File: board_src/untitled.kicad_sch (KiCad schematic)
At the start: 3 parts, among them J3 Conn_01x03, U5 DS18B20

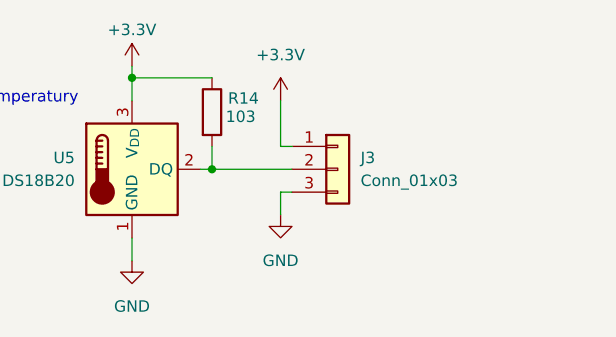
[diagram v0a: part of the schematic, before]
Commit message: Wersja początkowa 9.0
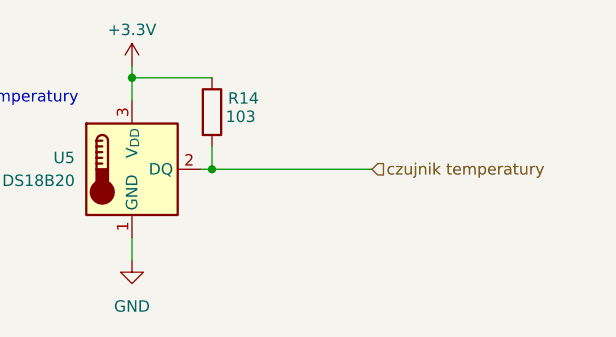
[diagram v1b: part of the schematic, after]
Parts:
- removed J3: Conn_01x03, symbol Connector_Generic:Conn_01x03
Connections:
- net czujnik temperatury: now reaches R14.2, U5.2 (DQ)
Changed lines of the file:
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@@
 	(wire
 		(pts
-			(xy 119.38 93.98) (xy 119.38 88.9)
-		)
-		(stroke
-			(width 0)
-			(type default)
-		)
-	)
-	(wire
-		(pts
-			(xy 120.65 99.06) (xy 119.38 99.06)
-		)
-		(stroke
-			(width 0)
-			(type default)
-		)
-	)
-	(wire
-		(pts
-			(xy 111.76 96.52) (xy 120.65 96.52)
+			(xy 111.76 96.52) (xy 129.54 96.52)
 		)
 		(stroke
@@
 	(wire
 		(pts
-			(xy 119.38 99.06) (xy 119.38 101.6)
-		)
-		(stroke
-			(width 0)
-			(type default)
-		)
-	)
-	(wire
-		(pts
-			(xy 120.65 93.98) (xy 119.38 93.98)
-		)
-		(stroke
-			(width 0)
-			(type default)
-		)
-	)
-	(wire
-		(pts
 			(xy 111.76 93.98) (xy 111.76 96.52)
 		)
@@
 			(width 0)
 			(type default)
+		)
+	)
+	(hierarchical_label "czujnik temperatury"
+		(shape input)
+		(at 129.54 96.52 0)
+		(effects
+			(font
+				(size 1.27 1.27)
+			)
+			(justify left)
 		)
 	)
@@
 	)
 	(symbol
-		(lib_id "Connector_Generic:Conn_01x03")
-		(at 125.73 96.52 0)
-		(unit 1)
-		(exclude_from_sim no)
-		(in_bom yes)
-		(on_board yes)
-		(dnp no)
-		(fields_autoplaced yes)
-		(property "Reference" "J3"
-			(at 128.27 95.2499 0)
-			(effects
-				(font
-					(size 1.27 1.27)
-				)
-				(justify left)
-			)
-		)
-		(property "Value" "Conn_01x03"
-			(at 128.27 97.7899 0)
-			(effects
-				(font
-					(size 1.27 1.27)
-				)
-				(justify left)
-			)
-		)
-		(property "Footprint" ""
-			(at 125.73 96.52 0)
-			(effects
-				(font
-					(size 1.27 1.27)
-				)
-				(hide yes)
-			)
-		)
-		(property "Datasheet" "~"
-			(at 125.73 96.52 0)
-			(effects
-				(font
-					(size 1.27 1.27)
-				)
-				(hide yes)
-			)
-		)
-		(property "Description" "Generic connector, single row, 01x03, script generated (kicad-library-utils/schlib/autogen/connector/)"
-			(at 125.73 96.52 0)
-			(effects
-				(font
-					(size 1.27 1.27)
-				)
-				(hide yes)
-			)
-		)
-		(pin "3"
-		)
-		(pin "2"
-		)
-		(pin "1"
-		)
-		(instances
-			(project "board"
-				(path "/772e9f49-cfcf-4cf6-843d-0684684f2d4b/4ce4dd53-34e3-426c-821d-561d412e5bd5"
-					(reference "J3")
-					(unit 1)
-				)
-			)
-		)
-	)
-	(symbol
 		(lib_id "power:GND")
 		(at 102.87 106.68 0)
@@
 					(unit 1)
 				)
-			)
-		)
-	)
-	(symbol
-		(lib_id "power:GND")
-		(at 119.38 101.6 0)
-		(unit 1)
-		(exclude_from_sim no)
-		(in_bom yes)
-		(on_board yes)
-		(dnp no)
-		(fields_autoplaced yes)
-		(property "Reference" "#PWR019"
-			(at 119.38 107.95 0)
-			(effects
-				(font
-					(size 1.27 1.27)
-				)
-				(hide yes)
-			)
-		)
-		(property "Value" "GND"
-			(at 119.38 106.68 0)
-			(effects
-				(font
-					(size 1.27 1.27)
-				)
-			)
-		)
-		(property "Footprint" ""
-			(at 119.38 101.6 0)
-			(effects
-				(font
-					(size 1.27 1.27)
-				)
-				(hide yes)
-			)
-		)
-		(property "Datasheet" ""
-			(at 119.38 101.6 0)
-			(effects
-				(font
-					(size 1.27 1.27)
-				)
-				(hide yes)
-			)
-		)
-		(property "Description" "Power symbol creates a global label with name \"GND\" , ground"
-			(at 119.38 101.6 0)
-			(effects
-				(font
-					(size 1.27 1.27)
-				)
-				(hide yes)
-			)
-		)
-		(pin "1"
-		)
-		(instances
-			(project "board"
-				(path "/772e9f49-cfcf-4cf6-843d-0684684f2d4b/4ce4dd53-34e3-426c-821d-561d412e5bd5"
-					(reference "#PWR019")
-					(unit 1)
-				)
-			)
-		)
-	)
-	(symbol
-		(lib_id "power:+3.3V")
-		(at 119.38 88.9 0)
-		(unit 1)
-		(exclude_from_sim no)
-		(in_bom yes)
-		(on_board yes)
-		(dnp no)
-		(fields_autoplaced yes)
-		(property "Reference" "#PWR018"
-			(at 119.38 92.71 0)
-			(effects
-				(font
-					(size 1.27 1.27)
-				)
-				(hide yes)
-			)
-		)
-		(property "Value" "+3.3V"
-			(at 119.38 83.82 0)
-			(effects
-				(font
-					(size 1.27 1.27)
-				)
-			)
-		)
-		(property "Footprint" ""
-			(at 119.38 88.9 0)
-			(effects
-				(font
-					(size 1.27 1.27)
-				)
-				(hide yes)
-			)
-		)
-		(property "Datasheet" ""
-			(at 119.38 88.9 0)
-			(effects
-				(font
-					(size 1.27 1.27)
-				)
-				(hide yes)
-			)
-		)
-		(property "Description" "Power symbol creates a global label with name \"+3.3V\""
-			(at 119.38 88.9 0)
-			(effects
-				(font
-					(size 1.27 1.27)
-				)
-				(hide yes)
-			)
-		)
-		(pin "1"
-		)
-		(instances
-			(project "board"
-				(path "/772e9f49-cfcf-4cf6-843d-0684684f2d4b/4ce4dd53-34e3-426c-821d-561d412e5bd5"
-					(reference "#PWR018")
-					(unit 1)
-				)

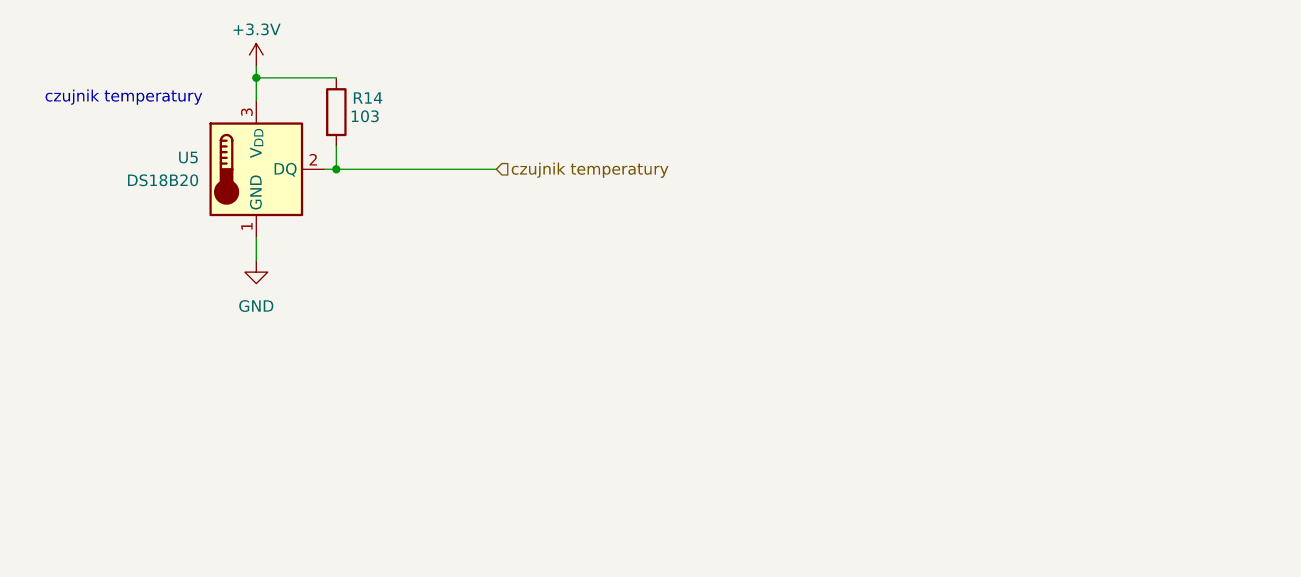
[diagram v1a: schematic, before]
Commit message: wersja dodane arkusze hierarchiczne
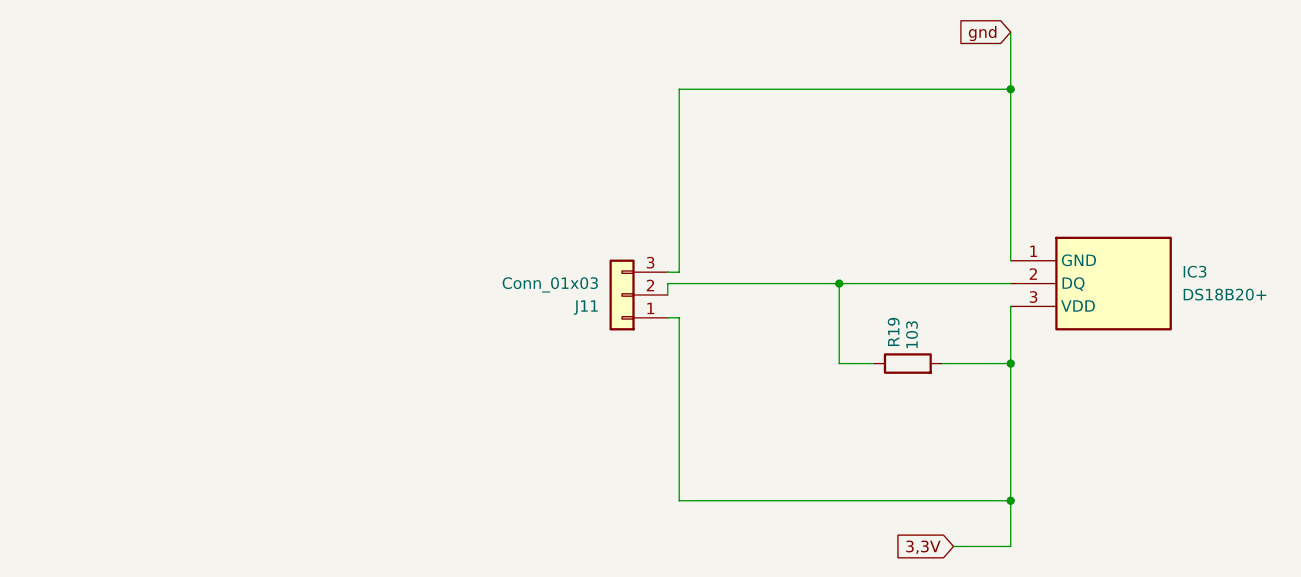
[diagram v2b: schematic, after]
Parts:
- removed R14: 103, Resistor_SMD:R_0201_0603Metric, symbol Device:R
- removed U5: DS18B20, Package_TO_SOT_THT:TO-92_Inline, symbol Sensor_Temperature:DS18B20
- added IC3: DS18B20+, DS18B20, symbol DS18B20+:DS18B20+
- added J11: Conn_01x03, symbol Connector_Generic:Conn_01x03
- added R19: 103, Resistor_SMD:R_0201_0603Metric, symbol Device:R
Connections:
- new net: IC3.2 (DQ), J11.2 (Pin_2), R19.1
- new net 3,3V: IC3.3 (VDD), J11.1 (Pin_1), R19.2
- new net gnd: IC3.1 (GND), J11.3 (Pin_3)
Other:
- note removed: "czujnik temperatury"
